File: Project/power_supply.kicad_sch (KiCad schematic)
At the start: 9 parts, among them U1 74LS04, U3 74LS08, U4 74LS32, U5 LM7805_TO220

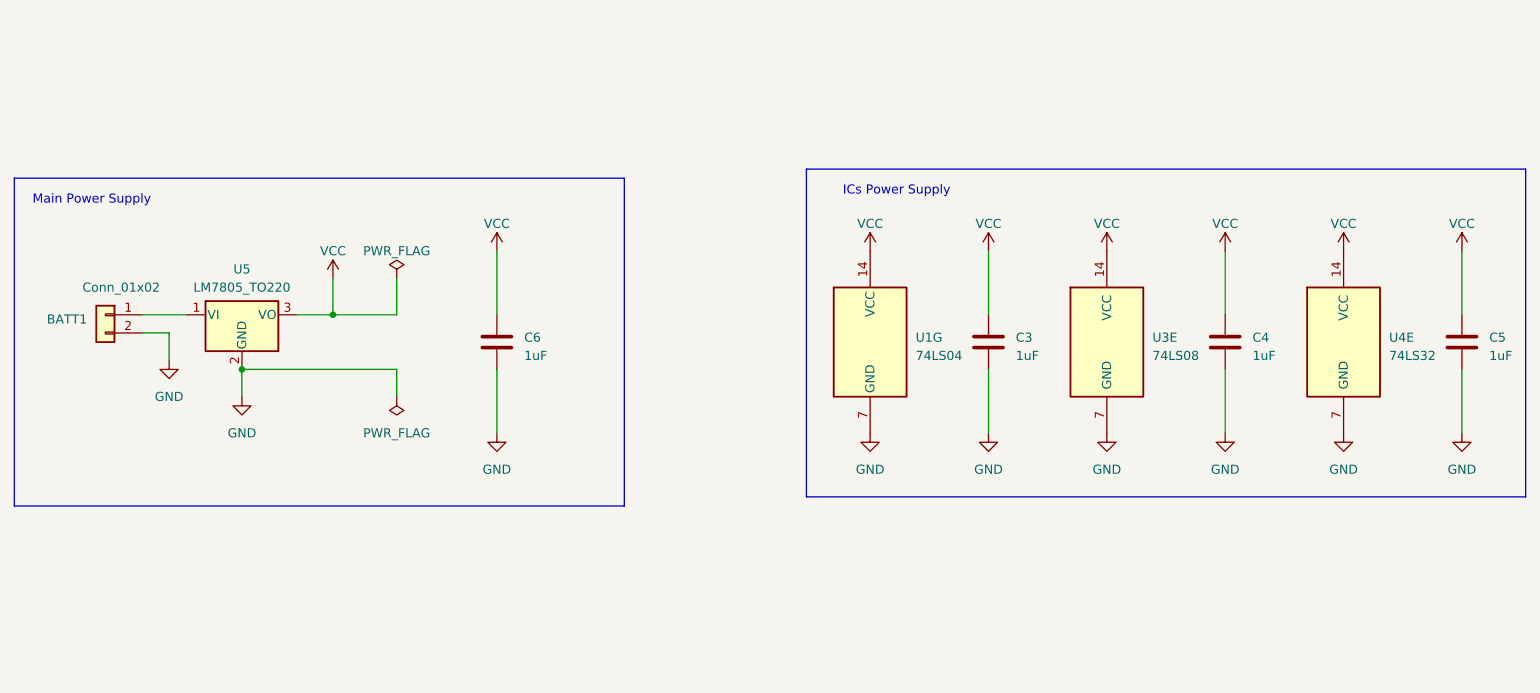
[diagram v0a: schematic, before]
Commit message: routing complete
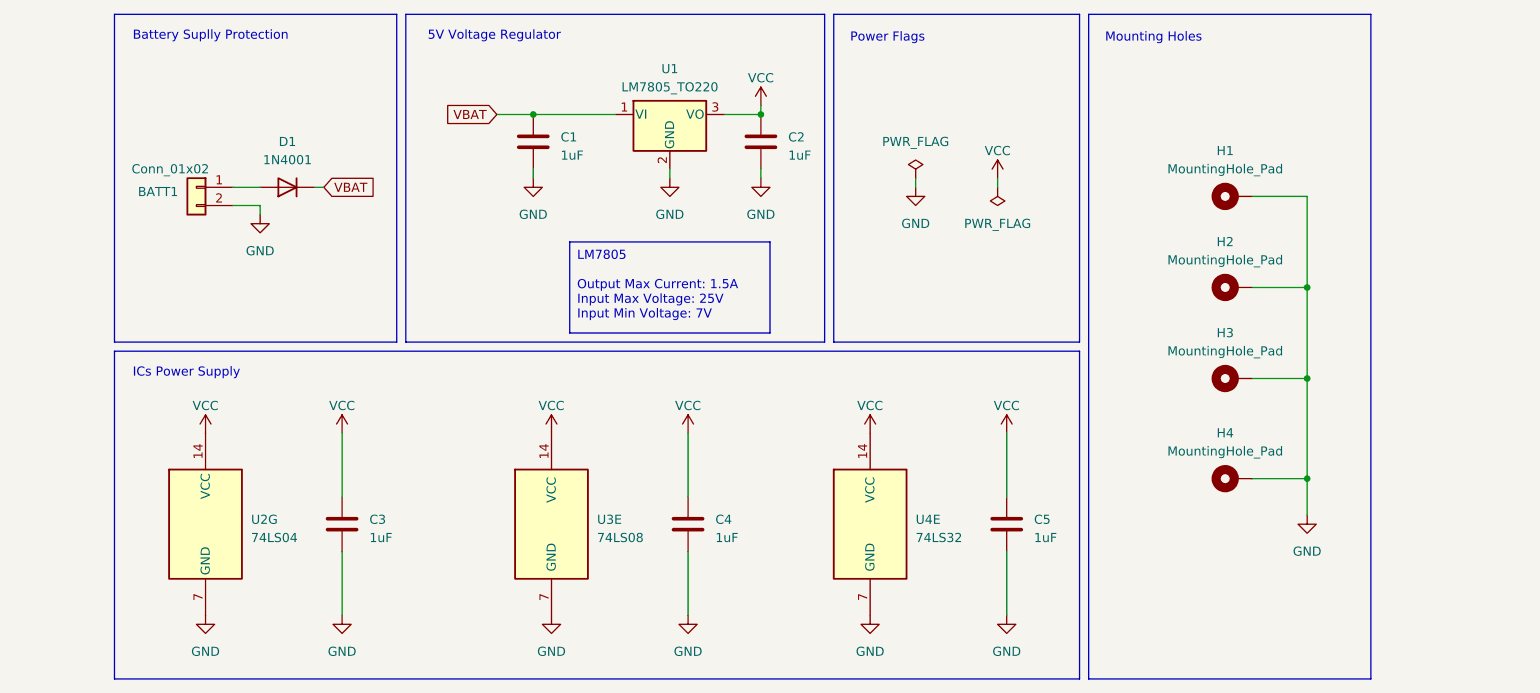
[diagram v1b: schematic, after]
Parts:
- removed C6: 1uF, Capacitor_THT:CP_Radial_D5.0mm_P2.50mm, symbol Device:C
- added C1, C2: 1uF, Capacitor_THT:CP_Radial_D5.0mm_P2.50mm, symbol Device:C
- added D1: 1N4001, Diode_THT:D_DO-41_SOD81_P10.16mm_Horizontal, symbol Diode:1N4001
- added H1, H2, H3, H4: MountingHole_Pad, MountingHole:MountingHole_4.3mm_M4_Pad_Via, symbol Mechanical:MountingHole_Pad
- U1: renamed from U5; footprint Package_TO_SOT_THT:TO-220-3_Vertical -> Package_TO_SOT_THT:TO-220-3_Horizontal_TabDown
- renumbered U1 to U2
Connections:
- net GND: now also C1.2, C2.2, H1.1, H2.1, H3.1, H4.1
- net VCC: now also C2.1
- net at BATT1.1 (Pin_1): now also D1.2 (A); no longer U1.1 (VI)
- new net VBAT: C1.1, D1.1 (K), U1.1 (VI)
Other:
- note added: "5V Voltage Regulator"
- note added: "Battery Suplly Protection"
- note added: "Mounting Holes"
- note added: "Power Flags"
- note removed: "Main Power Supply"
- company: (none) -> Marcos Yonamine
- title: (none) -> Digital Dice
- moved on the sheet: BATT1, C3, C4, C5, U1, U2G, U3E, U4E
